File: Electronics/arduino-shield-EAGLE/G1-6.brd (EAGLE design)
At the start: 53.7 x 68.3 mm, 23 parts

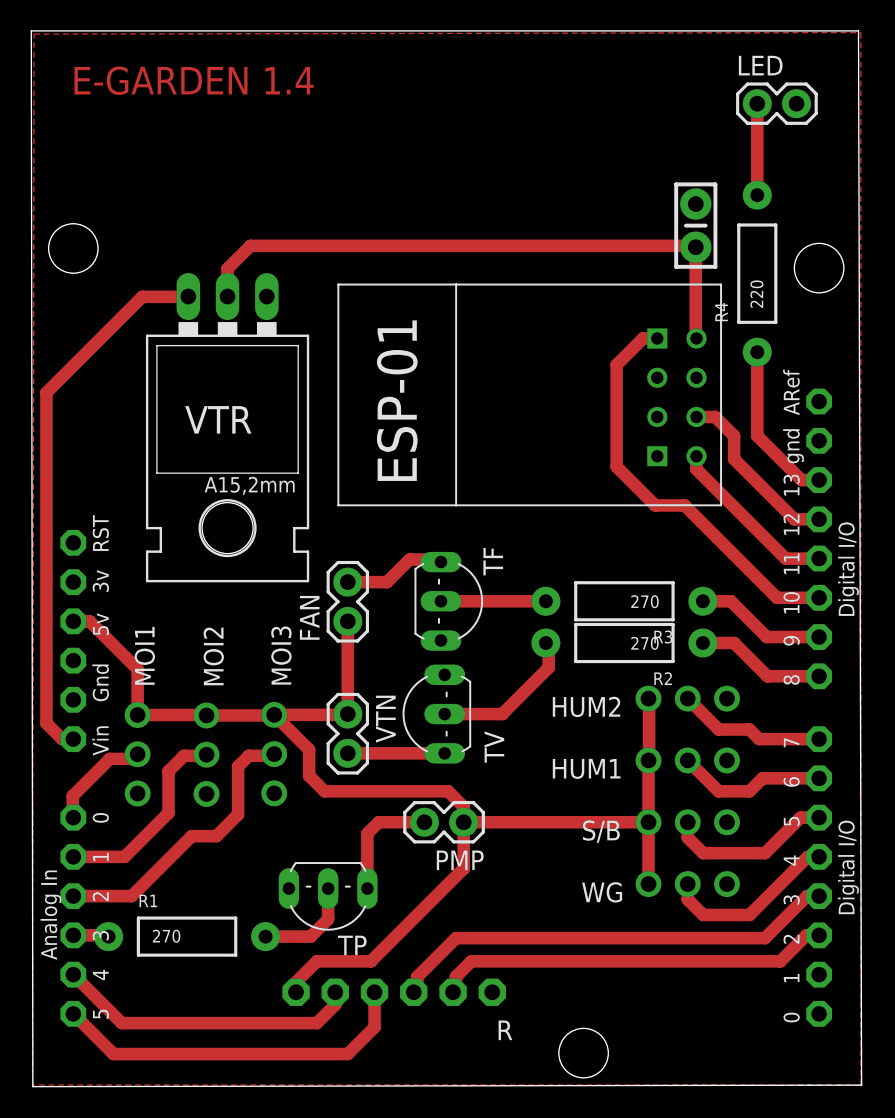
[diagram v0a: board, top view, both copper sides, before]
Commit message: shield version 1.6
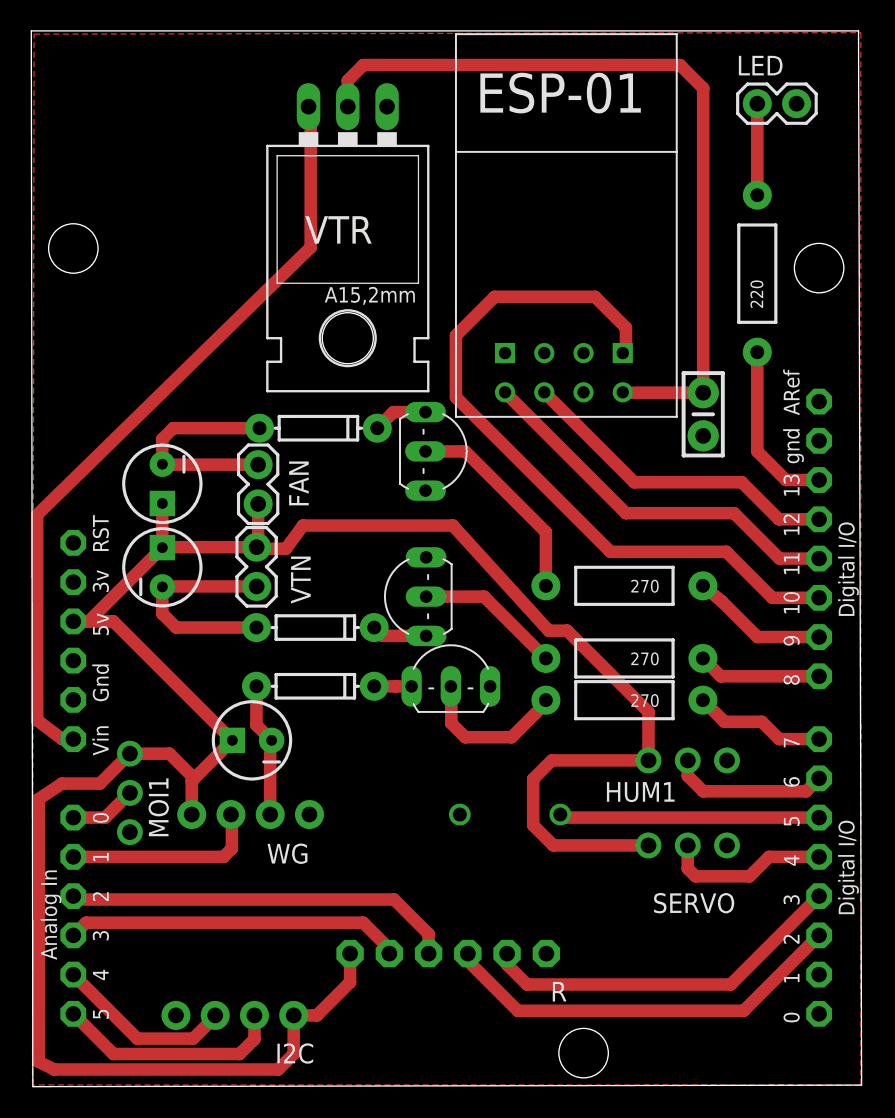
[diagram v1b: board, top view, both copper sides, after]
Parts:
- removed HUM2, MOI2, MOI3, S/B: (no value), adafruit:1X03-CLEANBIG
- removed PMP: (no value), SparkFun-Connectors:1X02
- added C2, C3, C4: (no value), SparkFun-Passives:CPOL-RADIAL-10UF-25V
- added D1, D2, D3: 1N4148, SparkFun-DiscreteSemi:DIODE-1N4148
- added I2C: (no value), SparkFun-Connectors:1X04_NO_SILK_ALL_ROUND
- added SERVO: (no value), adafruit:1X03-CLEANBIG
- added SG1: BUZZERNS, SparkFun-Electromechanical:BUZZER-12MM-NS
- WG: device adafruit:1X03-CLEANBIG -> SparkFun-Connectors:1X04_NO_SILK_ALL_ROUND
- moved WG 32.4 mm to (10.9, 18.5)
- moved R1 32.2 mm to (38.9, 25.9), turned to 180 degrees
- moved TP 17.5 mm to (27.7, 28.1), turned to 0 degrees
- moved VTR 14.5 mm to (21.0, 60.5)
- moved VTN 12.3 mm to (15.1, 35.8)
- moved C1 12.2 mm to (44.0, 44.4), turned to 90 degrees
- moved TF 9.75 mm to (27.3, 42.0)
- moved FAN 9.56 mm to (15.2, 38.6)
- moved U$2 8.50 mm to (35.0, 54.0), turned to 0 degrees
- moved TV 7.69 mm to (24.8, 32.6)
- moved R 4.30 mm to (27.5, 9.50)
- moved MOI1 2.55 mm to (6.90, 19.9)
- moved R2 1.00 mm to (38.9, 28.6)
- moved R3 1.00 mm to (38.9, 33.3)
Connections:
- removed net VTR: TV.E, VTN.2
- new net N$10: C4.2, D3.A, WG.3
- new net N$3: D2.C, TV.E
- new net N$6: C3.2, D2.A, VTN.2
- new net N$9: C2.2, D1.A, FAN.2
- net A1: now also WG.2; no longer MOI2.2
- net A2: now also R.4; no longer MOI3.2
- net A3: now also R.5; no longer R1.P$1
- net A4: now also I2C.3; no longer R.5
- net A5: now also I2C.2; no longer R.4
- net D2: now also R.3; no longer R.2
- net D3: now also R.2; no longer R.3
- net D4: now also SERVO.2; no longer WG.2
- net D5: now also SG1.+; no longer S/B.2
- net D7: now also R1.P$1; no longer HUM2.2
- net GND: now also I2C.4, SERVO.3, SG1.-, WG.4; no longer HUM2.3, MOI2.3, MOI3.3, S/B.3, WG.3
- net N$1: now also D1.C; no longer FAN.2
- net N$4: now also D3.C; no longer PMP.2
- net V5: now also C2.1, C3.1, C4.1, I2C.1, SERVO.1; no longer HUM2.1, MOI2.1, MOI3.1, PMP.1, S/B.1
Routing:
- net V5: track 86.3 -> 147.2 mm
- net D10: track 26.5 -> 47.5 mm
- net A3: track 2.31 -> 21.8 mm
- net V12: track 35.3 -> 50.0 mm
- net N$9: track 0.00 -> 14.5 mm
- net N$6: track 0.00 -> 14.3 mm
- net D11: track 11.2 -> 24.8 mm
- net N$8: track 38.7 -> 50.6 mm
- net D12: track 11.6 -> 21.2 mm
- net A5: track 23.6 -> 14.7 mm
- net N$10: track 0.00 -> 8.74 mm
- net A4: track 19.6 -> 11.6 mm
- net A2: track 18.6 -> 25.3 mm
- net N$5: track 6.79 -> 13.4 mm
- net VTR: track 6.27 -> 0.00 mm
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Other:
- board text removed: "E-GARDEN 1.4"
